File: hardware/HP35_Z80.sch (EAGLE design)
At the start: 82 parts, among them IC4 74HCT32N, IC5 74HCT154N, IC6 74HCT138N, IC7 74HCT541N, IC8 74HCT573N, IC9 74HCT573N, X1 MINI-USB-32005-301, X2 MINI-USB-32005-301

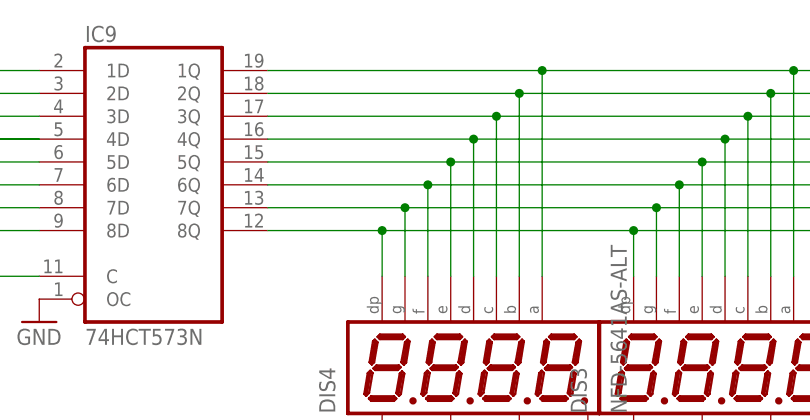
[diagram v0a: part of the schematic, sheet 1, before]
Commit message: update pcb
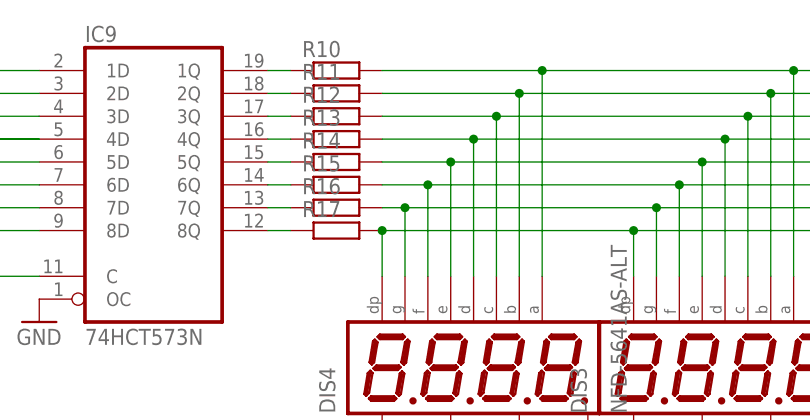
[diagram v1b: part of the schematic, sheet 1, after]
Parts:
- added R10, R11, R12, R13, R14, R15, R16, R17: (no value), rcl:R-EU_R1206
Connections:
- removed net N$35: DIS1.P$11, DIS2.P$11, DIS3.P$11, DIS4.P$11, IC9A.1Q
- new net N$10: IC9A.7Q, R16.1
- new net N$11: IC9A.6Q, R15.1
- new net N$12: IC9A.5Q, R14.1
- new net N$24: IC9A.4Q, R13.1
- new net N$25: IC9A.3Q, R12.1
- new net N$26: IC9A.2Q, R11.1
- new net N$27: IC9A.1Q, R10.1
- new net N$28: DIS1.P$11, DIS2.P$11, DIS3.P$11, DIS4.P$11, R10.2
- new net N$9: IC9A.8Q, R17.1
- net N$31: now also R17.2; no longer IC9A.8Q
- net N$32: now also R16.2; no longer IC9A.7Q
- net N$33: now also R15.2; no longer IC9A.6Q
- net N$34: now also R14.2; no longer IC9A.5Q
- net N$36: now also R11.2; no longer IC9A.2Q
- net N$37: now also R12.2; no longer IC9A.3Q
- net N$38: now also R13.2; no longer IC9A.4Q
